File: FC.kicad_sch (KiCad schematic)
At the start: 5 parts, among them U1 STM32H743VITx, U2 W25Q128JVS, U3 BMI270, U4 TPS7A20xxxDBV, U5 BMP280

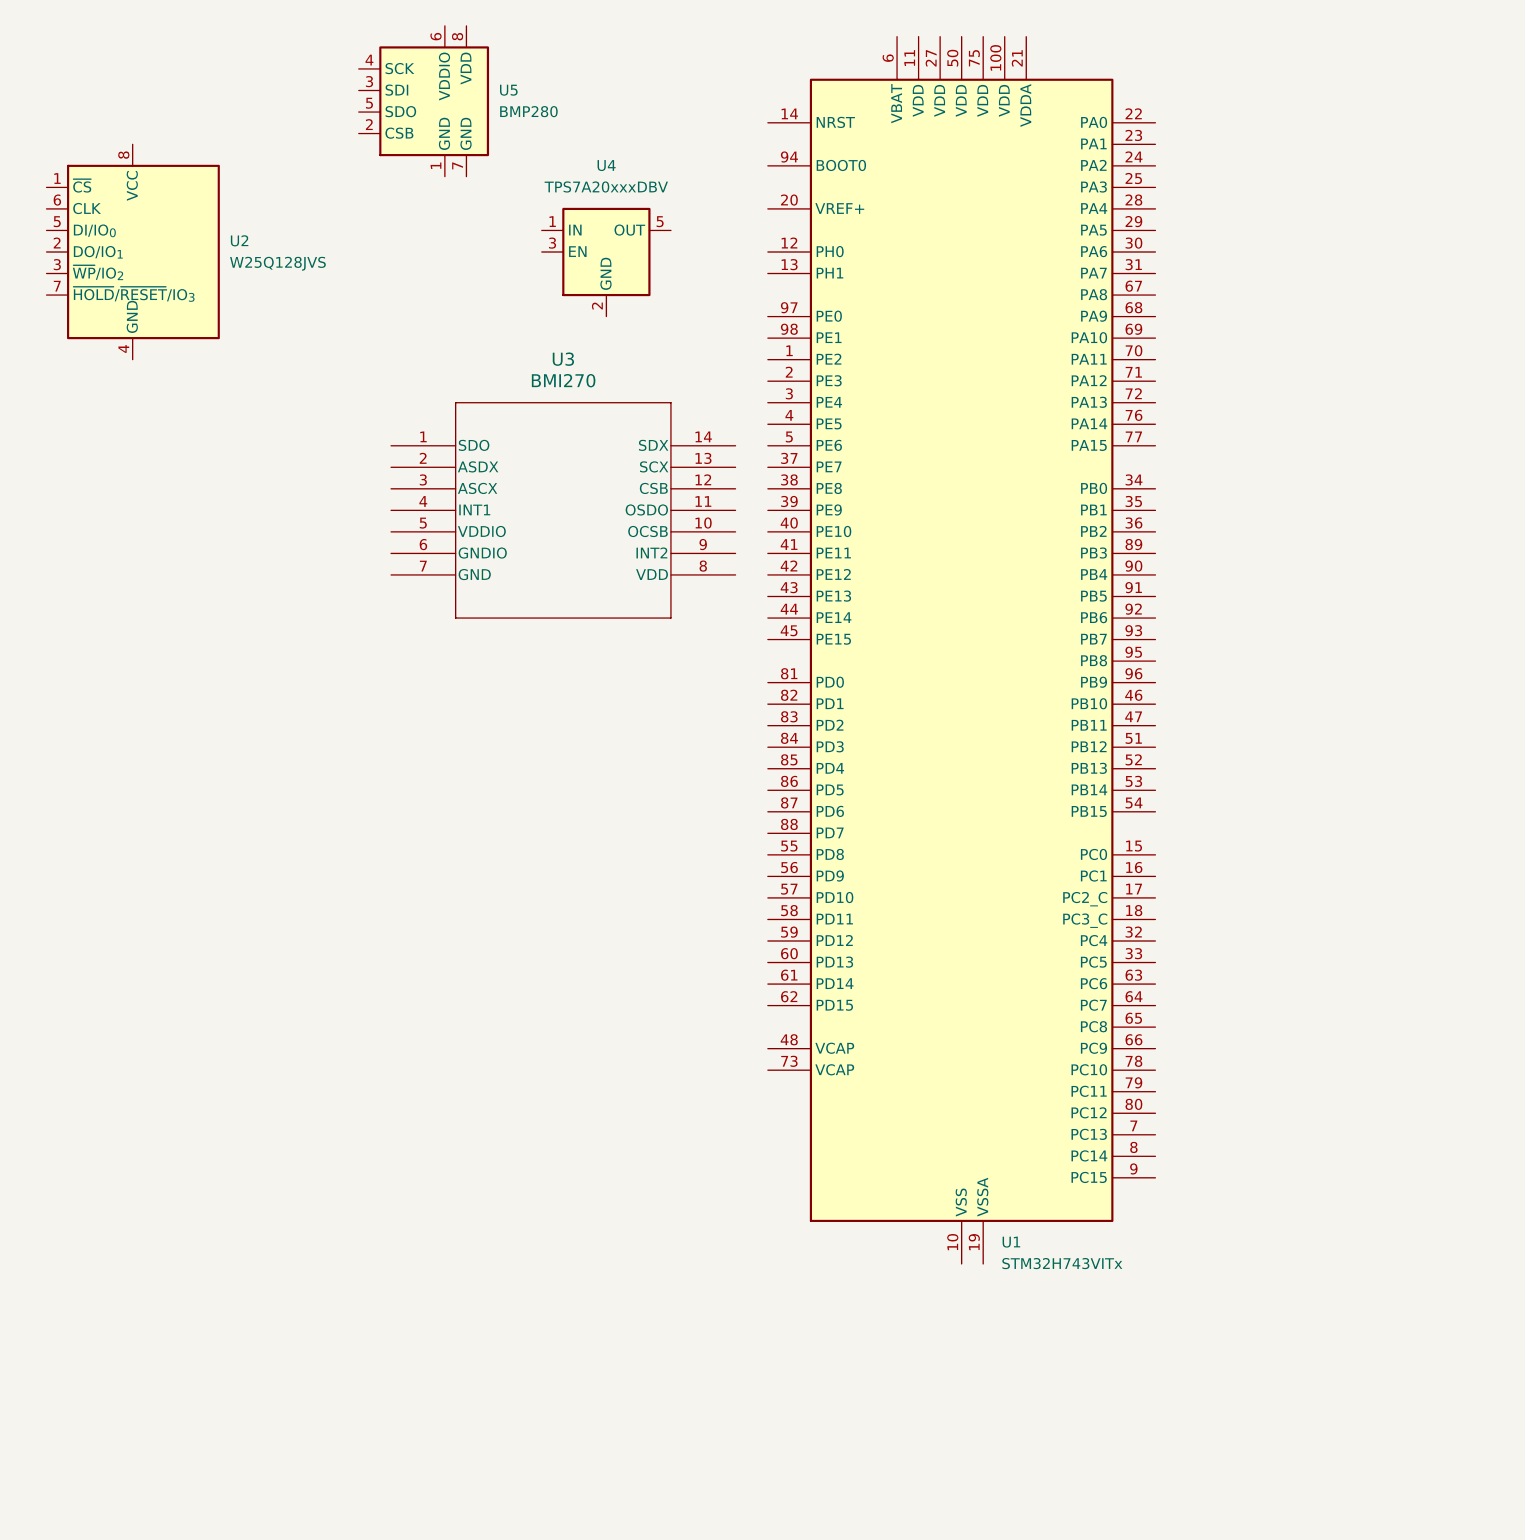
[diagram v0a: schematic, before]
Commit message: Power and reboot sys
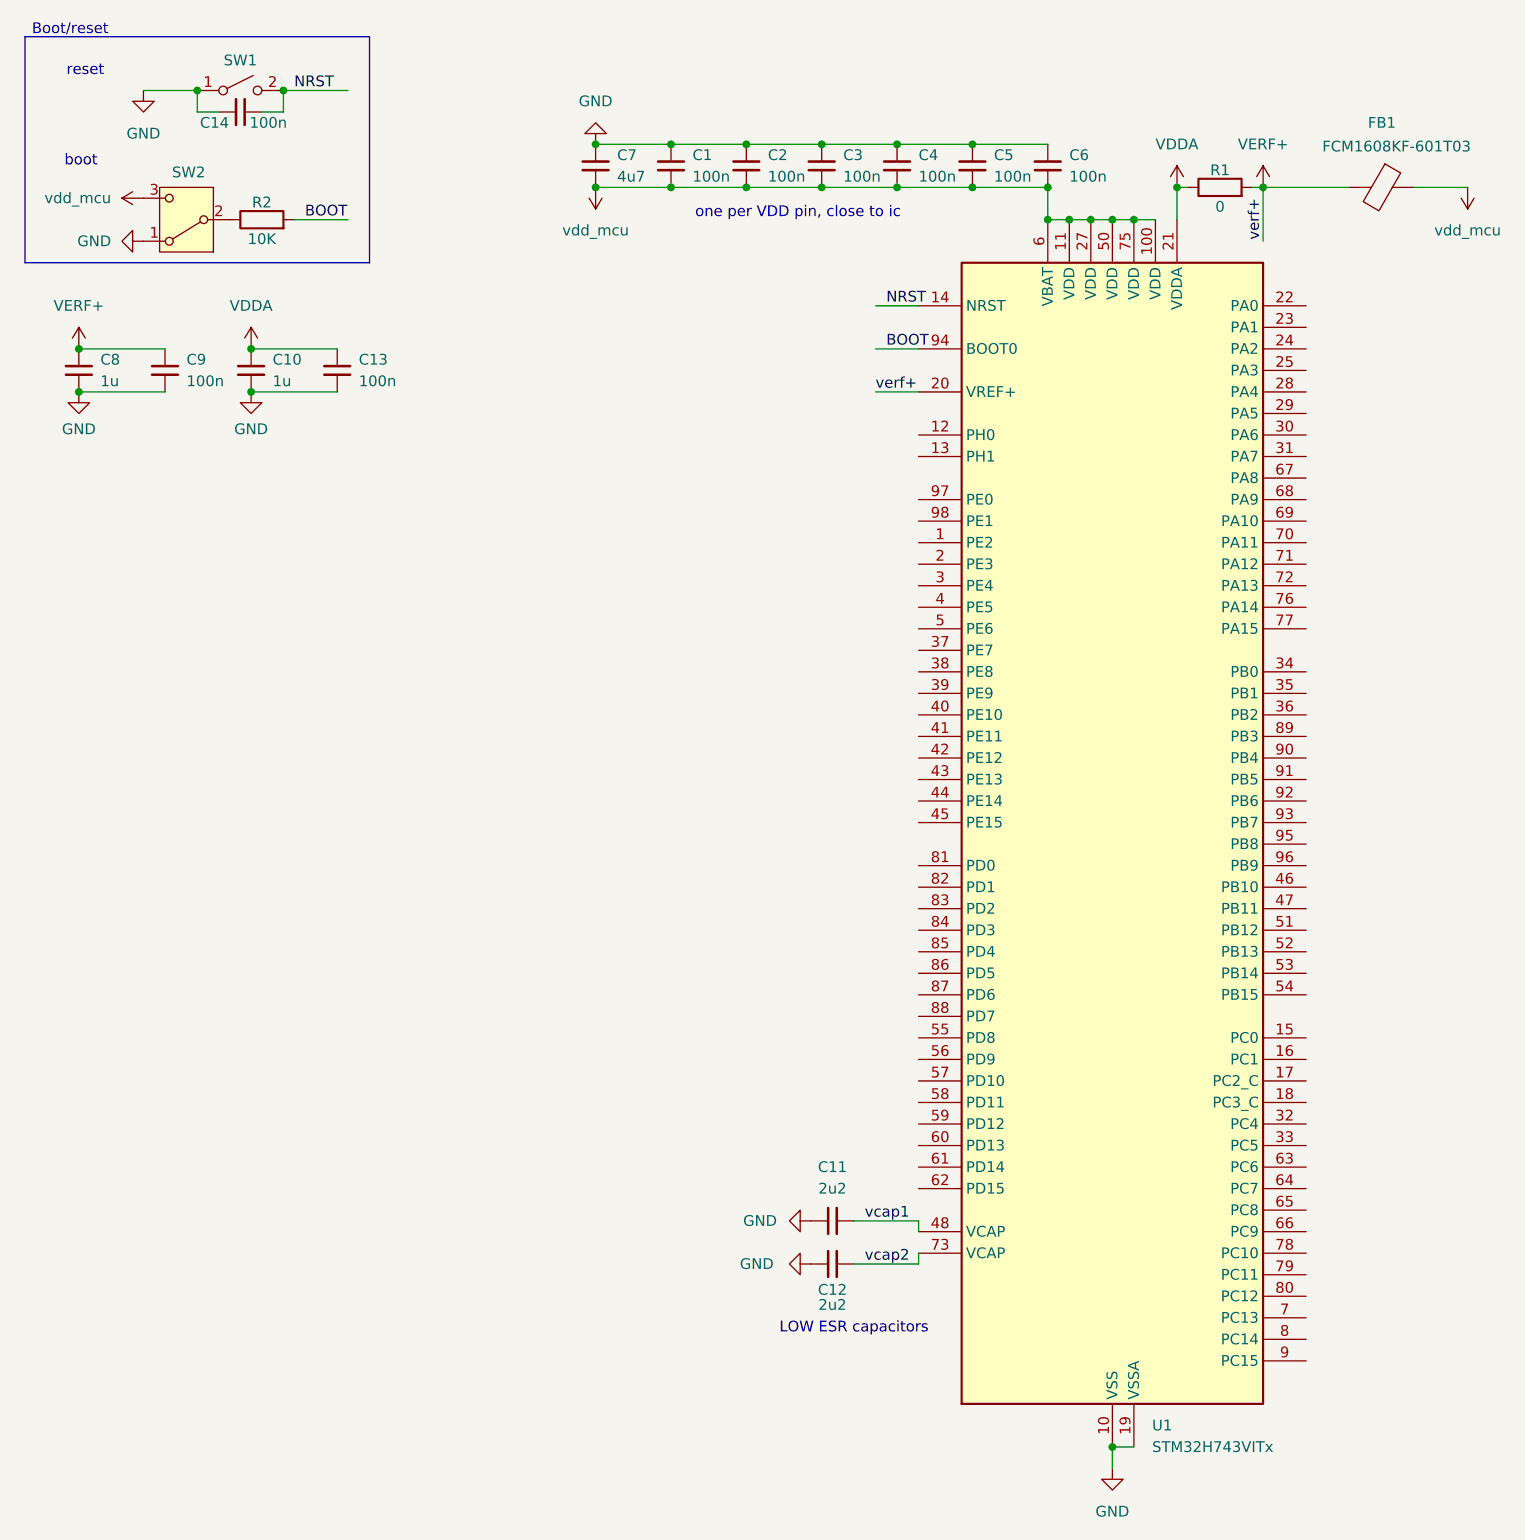
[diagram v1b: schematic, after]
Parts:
- removed U2: W25Q128JVS, Package_SO:SOIC-8_5.3x5.3mm_P1.27mm, symbol Memory_Flash:W25Q128JVS
- removed U3: BMI270, BMI270_BOS, symbol LIBRARY_SYM:BMI270
- removed U4: TPS7A20xxxDBV, Package_TO_SOT_SMD:SOT-23-5, symbol Regulator_Linear:TPS7A20xxxDBV
- removed U5: BMP280, Package_LGA:Bosch_LGA-8_2x2.5mm_P0.65mm_ClockwisePinNumbering, symbol Sensor_Pressure:BMP280
- added C1, C13, C14, C2, C3, C4, C5, C6, C9: 100n, Capacitor_SMD:C_0402_1005Metric, symbol Device:C_Small
- added C10, C8: 1u, Capacitor_SMD:C_0402_1005Metric, symbol Device:C_Small
- added C11, C12: 2u2, Capacitor_SMD:C_0402_1005Metric, symbol Device:C_Small
- added C7: 4u7, Capacitor_SMD:C_0402_1005Metric, symbol Device:C_Small
- added FB1: FCM1608KF-601T03, Package_LCC:PLCC-84_29.3x29.3mm_P1.27mm, symbol Device:FerriteBead
- added R1: 0, Package_DIP:DIP-8_W7.62mm, symbol Device:R
- added R2: 10K, Package_DIP:DIP-8_W7.62mm, symbol Device:R
- added SW1: SW_SPST, Button_Switch_THT:SW_NKK_NR01, symbol Switch:SW_SPST
- added SW2: SW_SPDT, symbol Switch:SW_SPDT
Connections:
- net GND: now reaches U1.10 (VSS), U1.26 (VSS), U1.49 (VSS), U1.74 (VSS), U1.99 (VSS)
- net GND: now also U1.19 (VSSA), C1.1, C10.2, C11.1, C12.1, C13.2, C14.1, C2.1, C3.1, C4.1, C5.1, C6.1, C7.1, C8.2, C9.2, SW1.1 (A), SW2.1 (A)
- net vdd_mcu: now reaches U1.100 (VDD)
- net vdd_mcu: now also U1.11 (VDD), U1.27 (VDD), U1.50 (VDD), U1.6 (VBAT), U1.75 (VDD), C1.2, C2.2, C3.2, C4.2, C5.2, C6.2, C7.2, FB1.1, SW2.3 (C)
- net NRST: now reaches U1.14 (NRST)
- net NRST: now also C14.2, SW1.2 (B)
- net VERF+: now reaches U1.20 (VREF+)
- net VERF+: now also C8.1, C9.1, FB1.2, R1.2
- net VDDA: now reaches U1.21 (VDDA)
- net VDDA: now also C10.1, C13.1, R1.1
- net vcap1: now reaches U1.48 (VCAP)
- net vcap1: now also C11.2
- net vcap2: now reaches U1.73 (VCAP)
- net vcap2: now also C12.2
- net BOOT: now reaches U1.94 (BOOT0)
- net BOOT: now also R2.2
- new net: R2.1, SW2.2 (B)
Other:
- note added: "Boot/reset"
- note added: "LOW ESR capacitors"
- note added: "boot"
- note added: "one per VDD pin, close to ic"
- note added: "reset"
- moved on the sheet: U1
